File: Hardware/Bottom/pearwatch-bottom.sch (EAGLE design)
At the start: 51 parts, among them SW1 SWITCH.MOM, SW2 SWITCH.MOM, U2 NRF52832_MODULE_MDBT42, U4 PCF8523

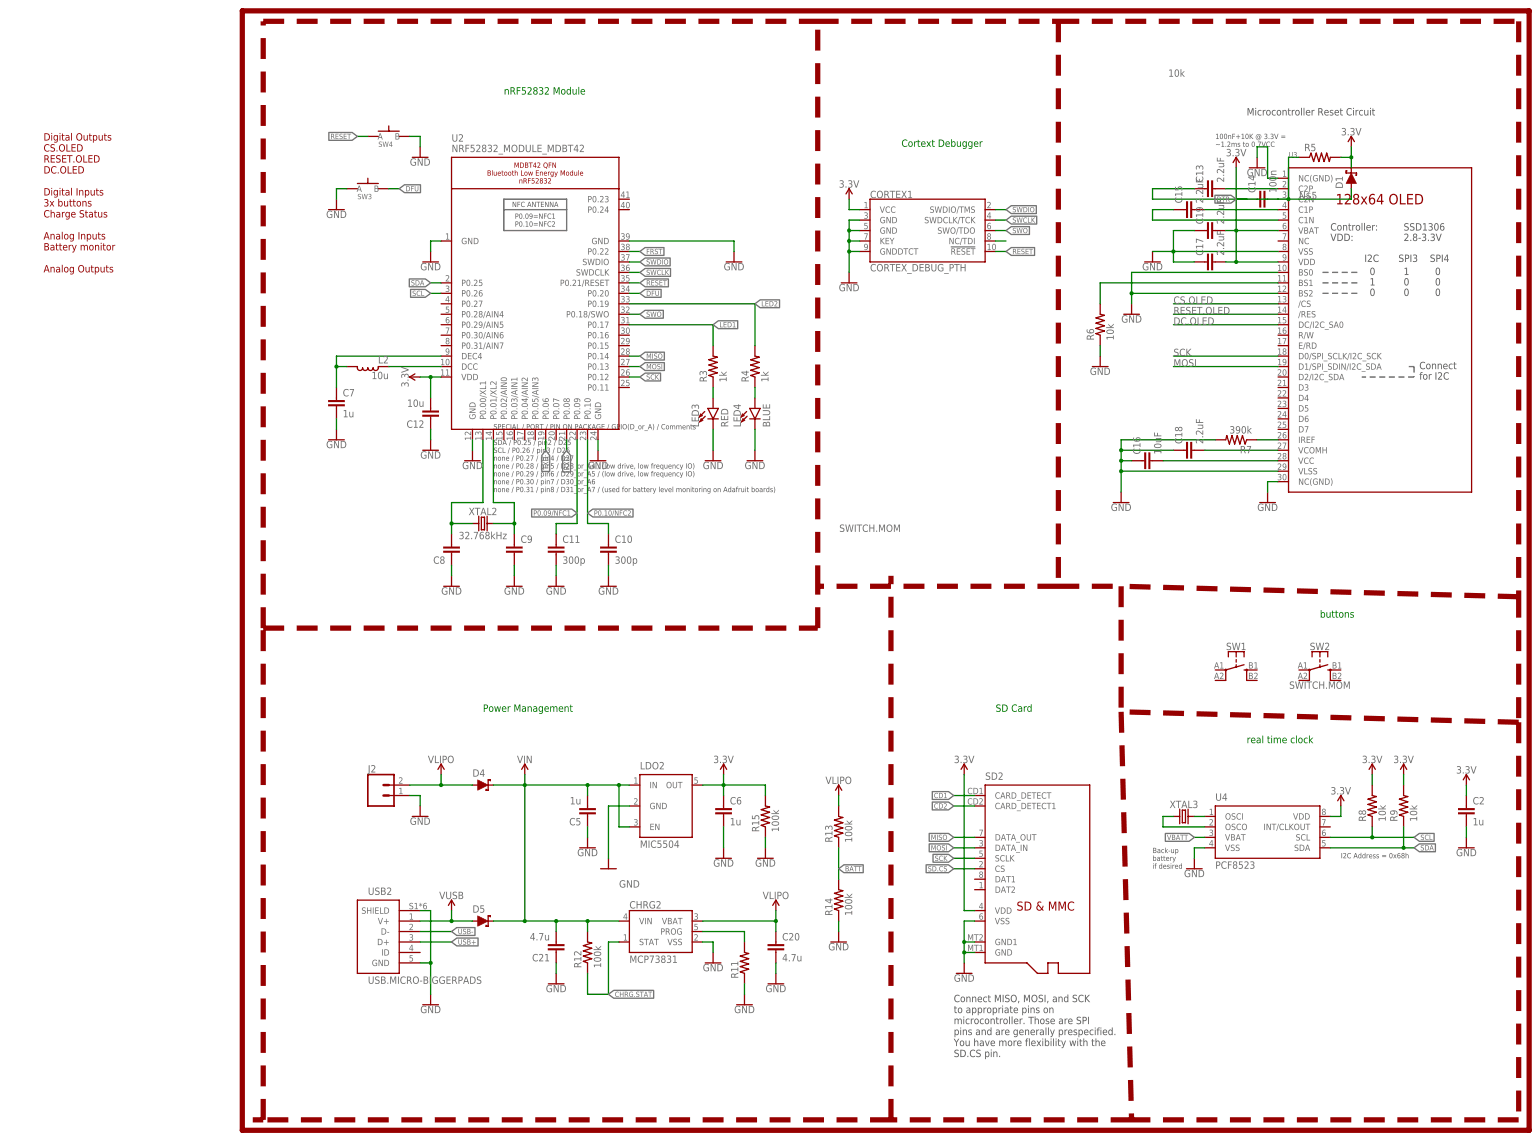
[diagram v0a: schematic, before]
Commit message: adding bottom board
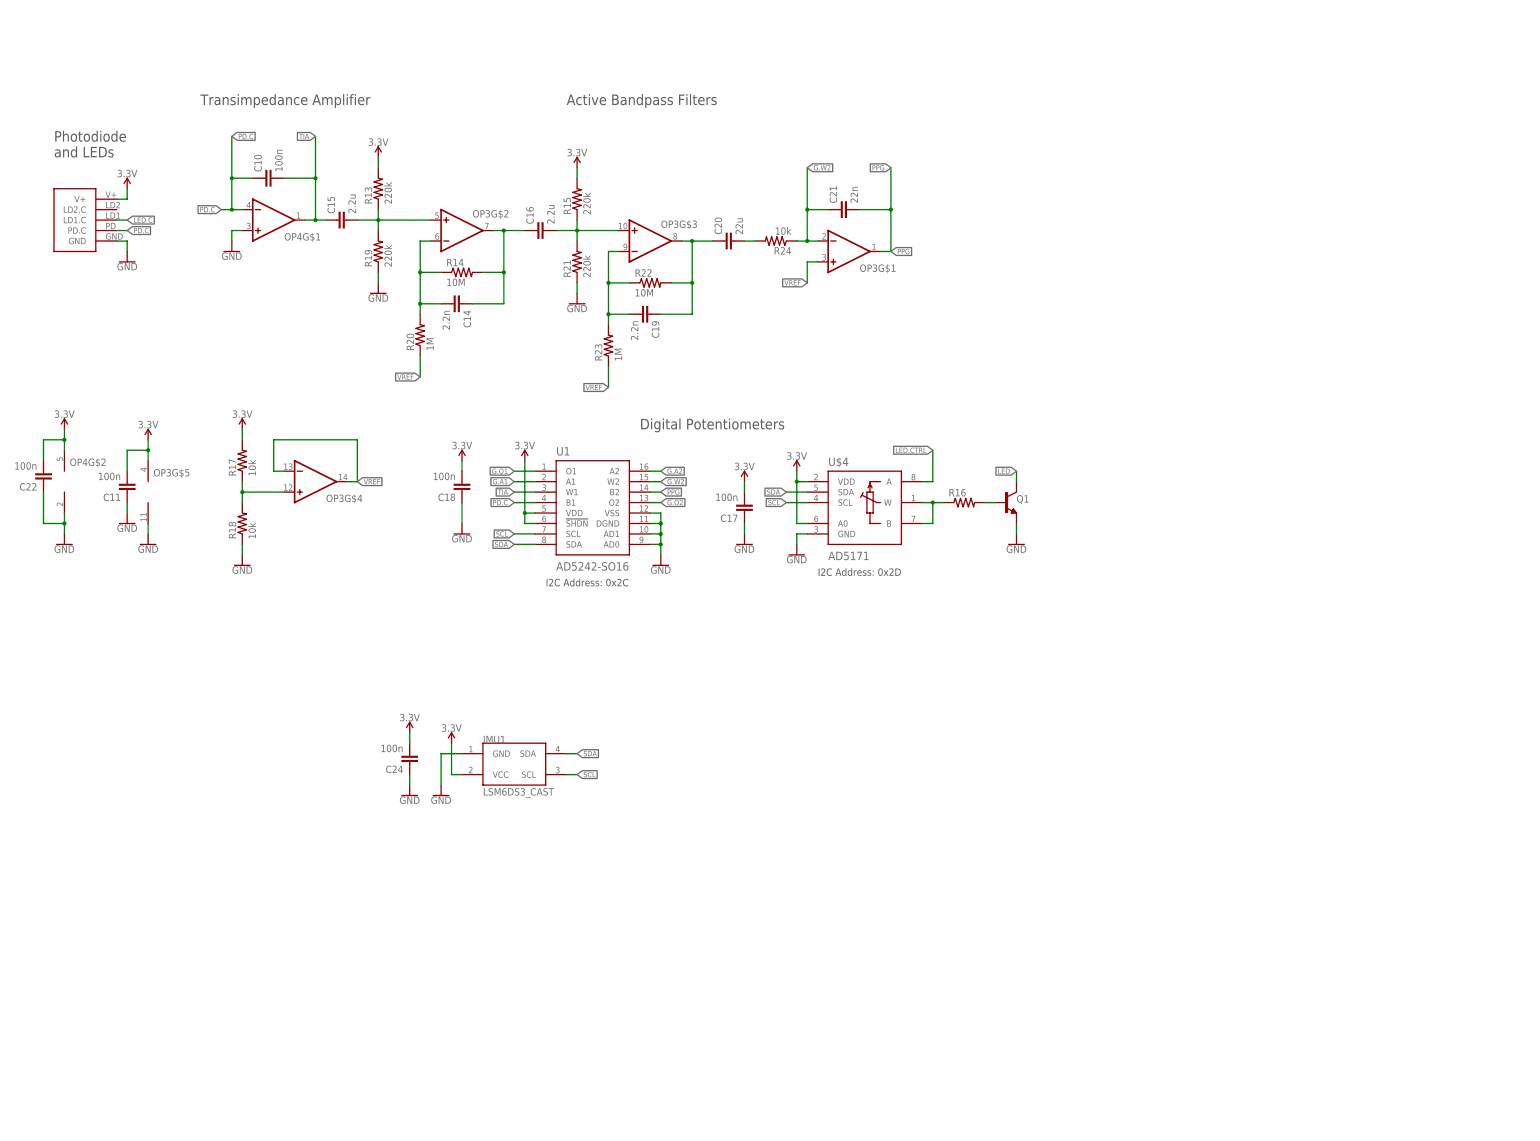
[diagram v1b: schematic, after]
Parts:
- removed C12: 10u, LinnesLab-Passives:CAPACITOR0805
- removed C13: 2.2uF, LinnesLab-Passives:CAPACITOR0402
- removed C2, C5, C6, C7: 1u, LinnesLab-Passives:CAPACITOR0603
- removed C8, C9: (no value), LinnesLab-Passives:CAPACITOR0603
- removed CHRG2: MCP73831, LinnesLab-Power:MCP73831
- removed CORTEX1: CORTEX_DEBUG_PTH, LinnesLab-Connectors:CORTEX_DEBUG_PTH
- removed D1, D4, D5: (no value), LinnesLab-DiscreteSemi:SCHOTTKY-USC
- removed J2: (no value), LinnesLab-Connectors:CONN_02
- removed L2: 10u, LinnesLab-Passives:INDUCTOR0603
- removed LDO2: MIC5504, LinnesLab-Power:MIC5504
- removed LED3: RED, LinnesLab-LED:LED0603
- removed LED4: BLUE, LinnesLab-LED:LED0603
- removed R11: (no value), LinnesLab-Passives:RESISTOR0603
- removed R12: 100k, LinnesLab-Passives:RESISTOR0603
- removed R3, R4: 1k, LinnesLab-Passives:RESISTOR0603
- removed R5, R6, R8, R9: 10k, LinnesLab-Passives:RESISTOR0603
- removed R7: 390k, LinnesLab-Passives:RESISTOR0603
- removed SD2: (no value), LinnesLab-Connectors:MICROSD
- removed SW1, SW2: SWITCH.MOM, LinnesLab-Switches:SWITCH.MOM
- removed SW3, SW4: (no value), LinnesLab-Switches:SPST-PTS830GG140-COPY.1-3
- removed U2: NRF52832_MODULE_MDBT42, LinnesLab-Microcontrollers:NRF52832_MODULE_MDBT42
- removed U3: (no value), LinnesLab-Displays:DISP_OLED_UG-2864HSWEG01-NO-WRAPAROUND
- removed U4: PCF8523, LinnesLab-Clocks:PCF8523
- removed USB2: USB.MICRO-BIGGERPADS, LinnesLab-Connectors:USB.MICRO-BIGGERPADS
- removed XTAL2: 32.768kHz, LinnesLab-Clocks:CRYSTALECS-.327-12.5-12-C-TR
- removed XTAL3: 32.7680kHz, LinnesLab-Clocks:CRYSTALECS-.327-12.5-12-C-TR
- added C22, C24: 100n, LinnesLab-Passives:CAPACITOR0603
- added IMU1: LSM6DS3_CAST, LinnesLab-Sensors:LSM6DS3_CAST
- added OP3: (no value), LinnesLab-AnalogIC:OP-QUAD-SO14
- added OP4: (no value), LinnesLab-AnalogIC:OP-SINGLEOT
- added Q1: (no value), LinnesLab-DiscreteSemi:NPN-GENERIC
- added R16: (no value), LinnesLab-Passives:RESISTOR0603
- added R17, R18: 10k, LinnesLab-Passives:RESISTOR0402
- added R19, R21: 220k, LinnesLab-Passives:RESISTOR0603
- added R20, R23: 1M, LinnesLab-Passives:RESISTOR0603
- added R22: 10M, LinnesLab-Passives:RESISTOR0603
- added R24: 10k, LinnesLab-Passives:RESISTOR0603
- added U$3: (no value), LinnesLab-Connectors:PPG.MODULE.2
- added U$4: AD5171, LinnesLab-DigitalIC:AD5171
- added U1: AD5242-SO16, LinnesLab-DigitalIC:AD5242-SO16
- C10, C11: value 300p -> 100n
- C14: value 100n -> 2.2n
- C15: value 2.2uF -> 2.2u; device LinnesLab-Passives:CAPACITOR0402 -> LinnesLab-Passives:CAPACITOR0603
- C16: value 10uF -> 2.2u
- C17, C18: value 2.2uF -> 100n; device LinnesLab-Passives:CAPACITOR0402 -> LinnesLab-Passives:CAPACITOR0603
- C19: value 2.2uF -> 2.2n; device LinnesLab-Passives:CAPACITOR0402 -> LinnesLab-Passives:CAPACITOR0603
- C20: value 4.7u -> 22u
- C21: value 4.7u -> 22n
- R13, R15: value 100k -> 220k
- R14: value 100k -> 10M
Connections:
- removed net BATT: R13.1, R14.2
- removed net CD1: SD2.CARD_DETECT
- removed net CD2: SD2.CARD_DETECT1
- removed net CHRG.STAT: CHRG2.STAT, R12.1
- removed net CS.OLED: U3./CS
- removed net DC.OLED: U3.DC/I2C_SA0
- removed net DFU: SW3.B, U2.P0.20
- removed net DTR: C14.1
- removed net FRST: U2.P0.22
- removed net LED1: R3.2, U2.P0.17
- removed net LED2: R4.2, U2.P0.19
- removed net MISO: SD2.DATA_OUT, U2.P0.14
- removed net MOSI: SD2.DATA_IN, U2.P0.13, U3.D1/SPI_SDIN/I2C_SDA
- removed net N$1: R6.2, U3.BS1
- removed net N$11: L2.1, U2.DCC
- removed net N$12: C7.1, L2.2, U2.DEC4
- removed net N$14: CORTEX1.NC/TDI
- removed net N$2: R7.1, U3.IREF
- removed net N$3: C13.2, U3.C2P
- removed net N$4: C8.2, U2.P0.00/XL1, XTAL2.1
- removed net N$5: C13.1, C14.2, D1.A, R5.1, U3.C2N
- removed net N$6: C9.1, U2.P0.01/XL2, XTAL2.2
- removed net N$7: C15.2, U3.C1P
- removed net P0.09/NFC1: C11.1, U2.P0.09
- removed net P0.10/NFC2: C10.1, U2.P0.10
- removed net RESET: CORTEX1.!RESET, SW4.A, U2.P0.21/RESET
- removed net RESET.OLED: U3./RES
- removed net RXD: U2.P0.08
- removed net SCK: SD2.SCLK, U2.P0.12, U3.D0/SPI_SCLK/I2C_SCK
- removed net SD.CS: SD2.CS
- removed net SWCLK: CORTEX1.SWDCLK/TCK, U2.SWDCLK
- removed net SWDIO: CORTEX1.SWDIO/TMS, U2.SWDIO
- removed net SWO: CORTEX1.SWO/TDO, U2.P0.18/SWO
- removed net TXD: U2.P0.06
- removed net USB+: USB2.D+
- removed net USB-: USB2.D-
- removed net VBATT: U4.VBAT
- removed net VIN: C21.2, C5.2, CHRG2.VIN, D4.C, D5.C, LDO2.EN, LDO2.IN, R12.2
- removed net VLIPO: C20.1, CHRG2.VBAT, D4.A, J2.2, R13.2
- removed net V_USB: D5.A, USB2.V+
- new net G.A1: U1.A1
- new net G.A2: U1.A2
- new net G.O1: U1.O1
- new net G.O2: U1.O2
- new net G.W2: C21.1, OP3G$1.-IN, R24.1, U1.W2
- new net LED: Q1.C
- new net LED.C: U$3.LD1.C
- new net LED.CTRL: U$4.A
- new net N$16: C14.1, C16.1, OP3G$2.OUT, R14.2
- new net N$18: C19.2, OP3G$3.-IN, R22.1, R23.2
- new net PD.C: C10.1, OP4G$1.-IN, U$3.PD.C, U1.B1
- new net PPG: C21.2, OP3G$1.OUT, U1.B2
- new net TIA: C10.2, C15.1, OP4G$1.OUT, U1.W1
- new net VREF: OP3G$1.+IN, OP3G$4.-IN, OP3G$4.OUT, R20.1, R23.1
- net 3.3V: now also C11.2, C18.2, C22.2, C24.2, IMU1.VCC, OP3G$5.V+, OP4G$2.V+, R13.2, R17.2, U$3.V+, U$4.A0, U$4.VDD, U1.!SHDN, U1.VDD; no longer C12.2, C19.2, C2.1, C6.1, CORTEX1.VCC, D1.C, LDO2.OUT, R5.2, R8.2, R9.2, SD2.VDD, U2.VDD, U3.VBAT, U3.VDD, U4.VDD
- net GND: now also C11.1, C22.1, C24.1, IMU1.GND, OP3G$5.V-, OP4G$1.+IN, OP4G$2.V-, Q1.E, R18.1, R19.1, R21.1, U$3.GND, U$4.GND, U1.AD0, U1.AD1, U1.DGND, U1.VSS; no longer C10.2, C11.2, C12.1, C16.1, C19.1, C2.2, C20.2, C21.1, C5.1, C6.2, C7.2, C8.1, C9.2, CHRG2.VSS, CORTEX1.GND@3, CORTEX1.GND@5, CORTEX1.GNDDTCT, CORTEX1.KEY, J2.1, LDO2.GND, LED3.C, LED4.C, R11.1, R14.1, R15.1, R6.1, R7.2, SD2.GND, SD2.GND1, SD2.VSS, SW3.A, SW4.B, U2.GND@1, U2.GND@2, U2.GND@3, U2.GND@4, U3.BS0, U3.BS2, U3.NC(GND)@1, U3.NC(GND)@2, U3.VLSS, U3.VSS, U4.VSS, USB2.GND, USB2.SHIELD
- net N$10: now also OP3G$4.+IN, R17.1, R18.2; no longer LED4.A, R4.1
- net N$13: now also C15.2, OP3G$2.+IN, R13.1, R19.2; no longer C16.2, U3.VCC
- net N$15: now also C14.2, OP3G$2.-IN, R14.1, R20.2; no longer C18.2, U3.VCOMH
- net N$17: now also C16.2, OP3G$3.+IN, R15.1, R21.2; no longer CHRG2.PROG, R11.2
- net N$19: now also C19.1, C20.1, OP3G$3.OUT, R22.2; no longer U4.OSCO, XTAL3.1
- net N$20: now also C20.2, R24.2; no longer U4.OSCI, XTAL3.2
- net N$8: now also Q1.B, R16.2; no longer C15.1, U3.C1N
- net N$9: now also R16.1, U$4.B, U$4.W; no longer LED3.A, R3.1
- net SCL: now also IMU1.SCL, U$4.SCL, U1.SCL; no longer R8.1, U2.P0.26, U4.SCL
- net SDA: now also IMU1.SDA, U$4.SDA, U1.SDA; no longer R9.1, U2.P0.25, U4.SDA
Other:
- note added: "Active Bandpass Filters"
- note added: "Digital Potentiometers"
- note added: "I2C Address: 0x2C"
- note added: "I2C Address: 0x2D"
- note added: "Photodiode and LEDs"
- note added: "Transimpedance Amplifier"
- note removed: "100nF+10K @ 3.3V = ~1.2ms to 0.7VCC"
- note removed: "Back-up battery if desired"
- note removed: "Connect MISO, MOSI, and SCK to appropriate pins on microcontroller. Those are SPI pins and are generally prespecified. You have more flexibility with the SD.CS pin."
- note removed: "Cortext Debugger"
- note removed: "Digital Outputs CS.OLED RESET.OLED DC.OLED Digital Inputs 3x buttons Charge Status Analog Inputs Battery monitor Analog Outputs"
- note removed: "I2C Address = 0x68h"
- note removed: "Microcontroller Reset Circuit"
- note removed: "OLED"
- note removed: "Power Management"
- note removed: "SD Card"
- note removed: "SPECIAL / PORT / PIN ON PACKAGE / GPIO(D_or_A) / Comments SDA / P0.25 / pin2 / D25 SCL / P0.26 / pin3 / D26 none / P0.27 / pin4 / D27 none / P0.28 / pin5 / D28_or_A4 / (low drive, low frequency IO) none / P0.29 / pin6 / D29_or_A5 / (low drive, low frequency IO) none / P0.30 / pin7 / D30_or_A6 none / P0.31 / pin8 / D31_or_A7 / (used for battery level monitoring on Adafruit boards)"
- note removed: "buttons"
- note removed: "nRF52832 Module"
- note removed: "real time clock"
- moved on the sheet: C10, C11, C14, C15, C16, C17, C18, C19, C20, C21, R13, R14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
